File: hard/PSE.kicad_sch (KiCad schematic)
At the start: 4 parts

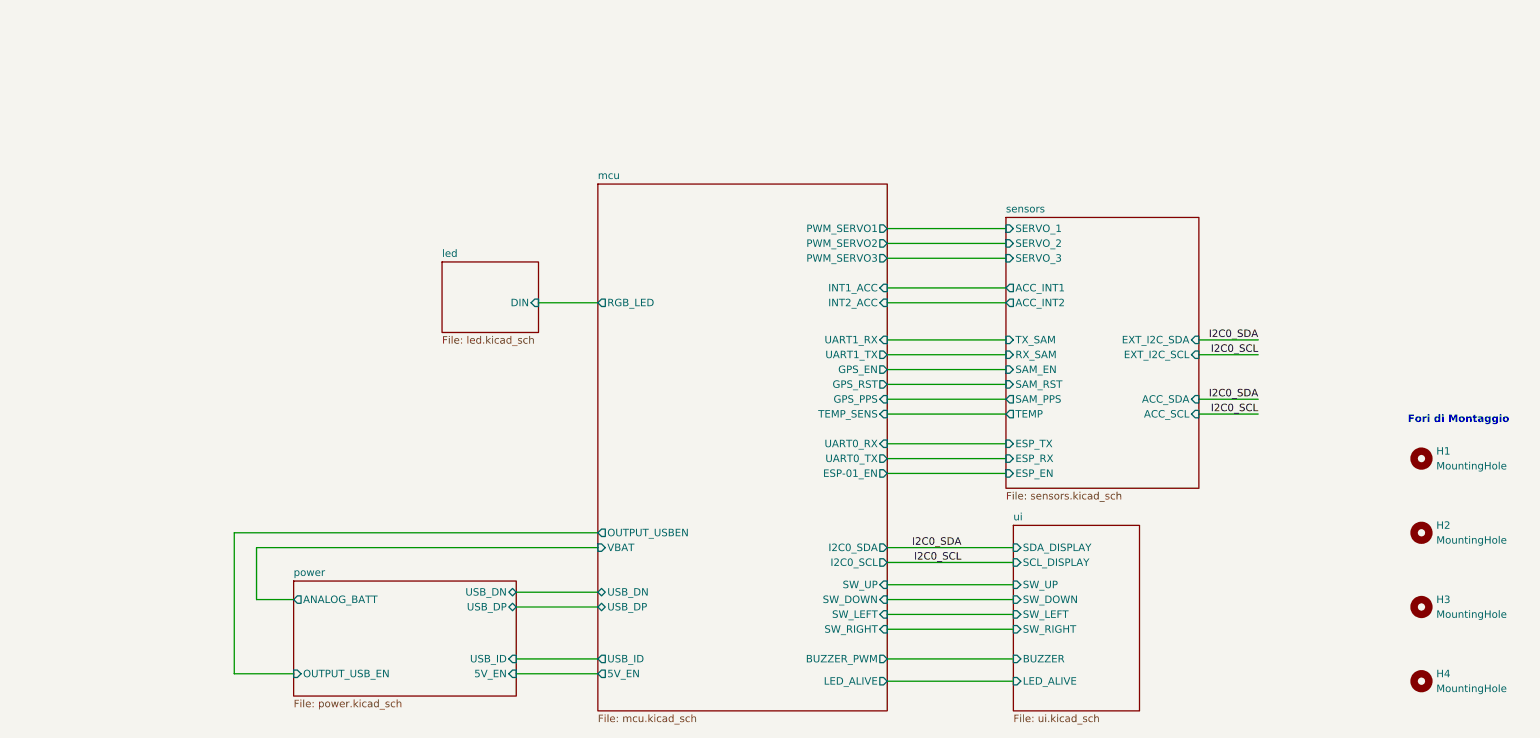
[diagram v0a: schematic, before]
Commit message: update
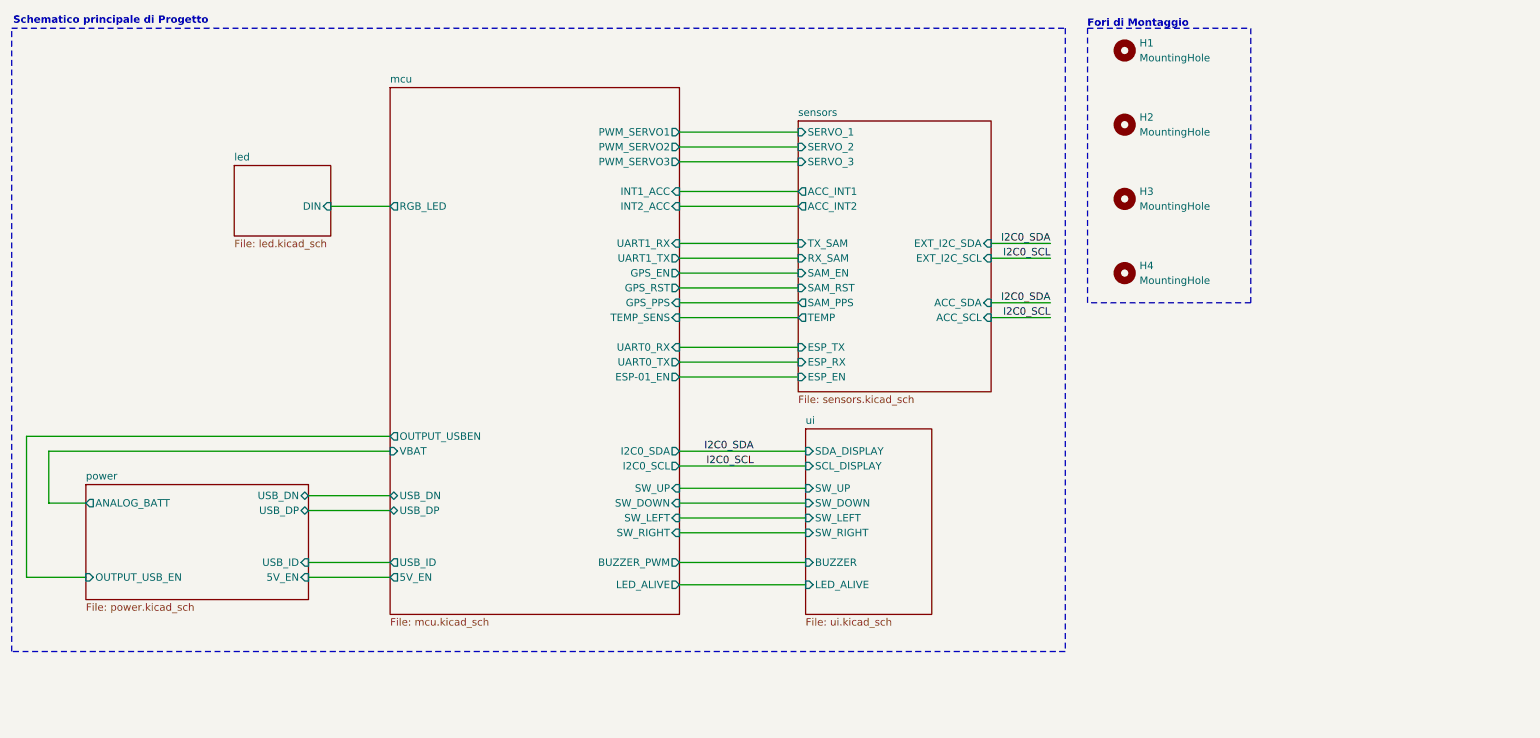
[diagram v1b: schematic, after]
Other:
- note added: "Schematico principale di Progetto"
- company: Universita' di Trento -> Universita' di Trento - DISI
- title: PSE -> Progettazione e Prototipazione di Sistemi Elettronici
- moved on the sheet: H1, H2, H3, H4
